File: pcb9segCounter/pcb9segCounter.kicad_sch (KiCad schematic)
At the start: 0 parts

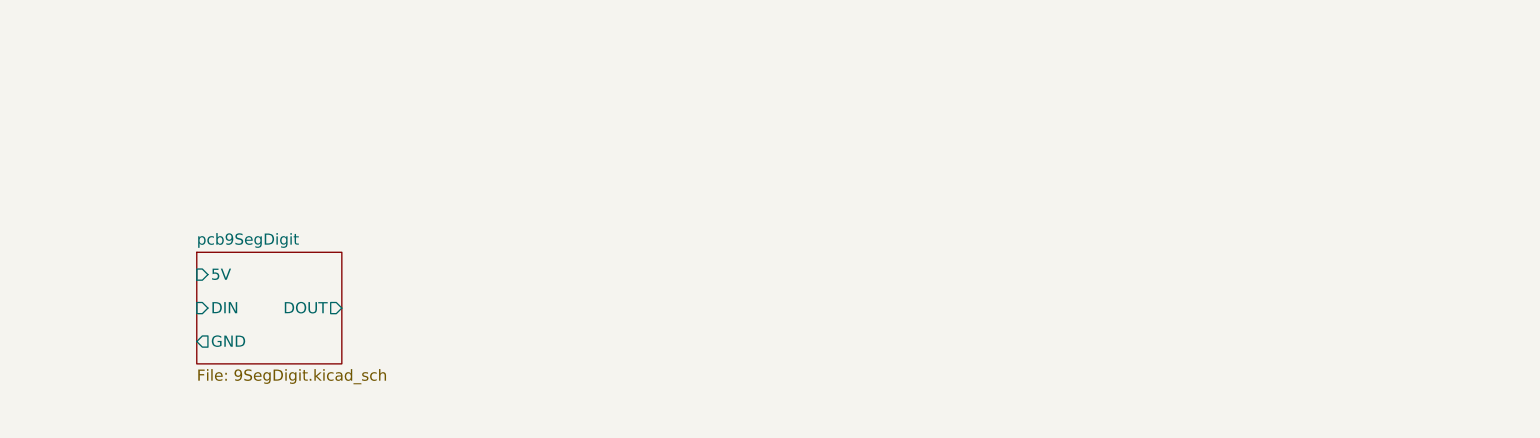
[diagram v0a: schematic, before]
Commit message: Making progress, figuring out microcontroller interfacing
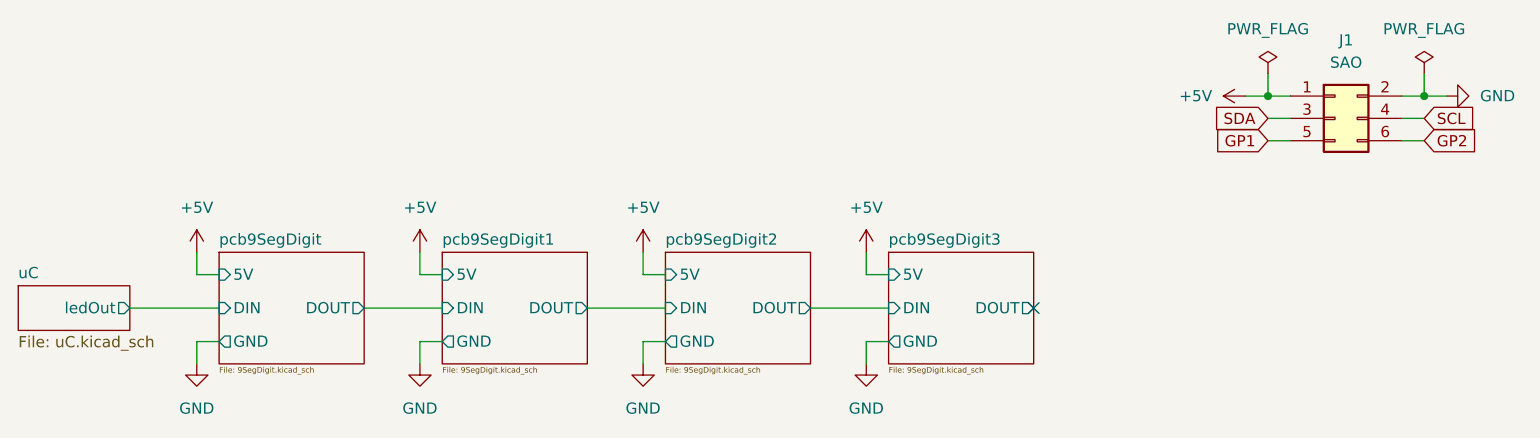
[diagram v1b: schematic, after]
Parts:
- added J1: SAO, Connector_PinHeader_2.54mm:PinHeader_2x03_P2.54mm_Vertical, symbol Connector_Generic:Conn_02x03_Odd_Even
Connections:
- new net +5V: J1.1 (Pin_1)
- new net GND: J1.2 (Pin_2)
- new net GP1: J1.5 (Pin_5)
- new net GP2: J1.6 (Pin_6)
- new net SCL: J1.4 (Pin_4)
- new net SDA: J1.3 (Pin_3)
- no-connect marks 0 -> 1
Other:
- added sheet pcb9SegDigit1 (9SegDigit.kicad_sch)
- added sheet pcb9SegDigit2 (9SegDigit.kicad_sch)
- added sheet pcb9SegDigit3 (9SegDigit.kicad_sch)
- added sheet uC (uC.kicad_sch)
